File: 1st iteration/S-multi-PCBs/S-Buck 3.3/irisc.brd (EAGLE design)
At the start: 38.9 x 32.8 mm, 18 parts

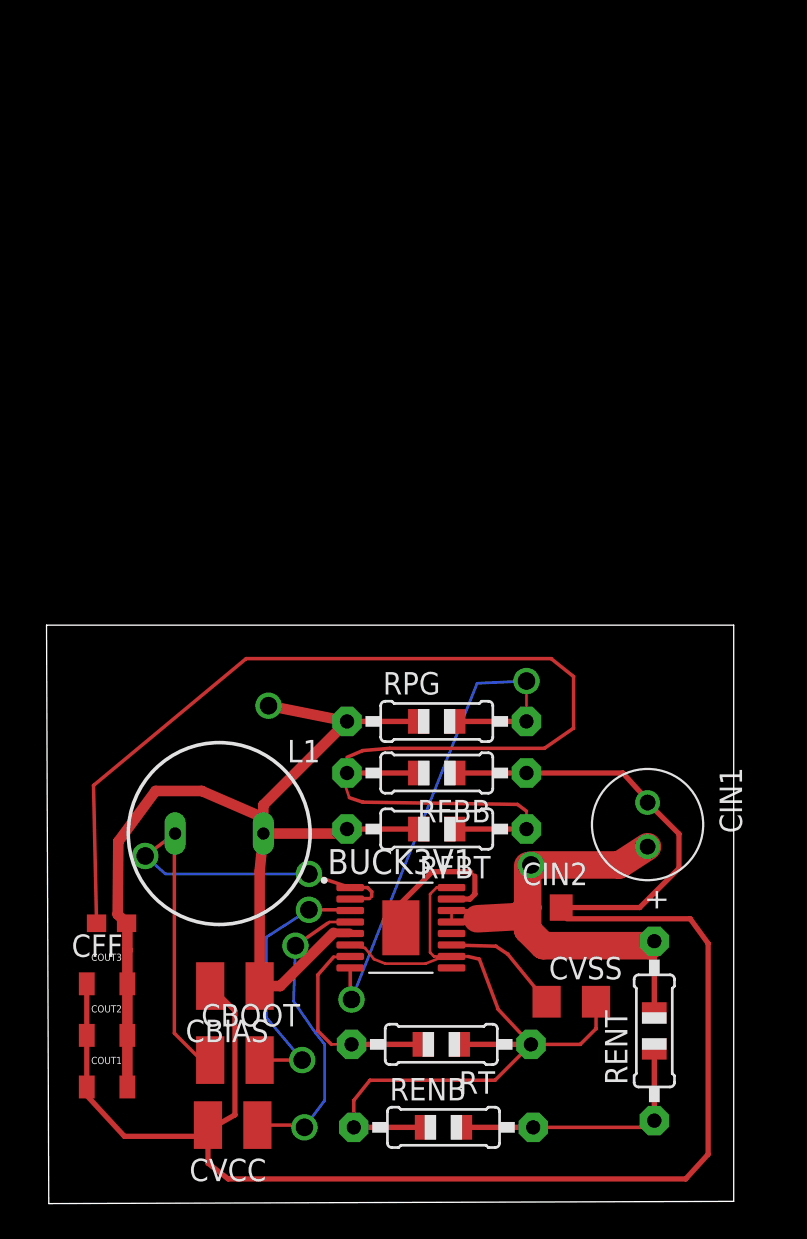
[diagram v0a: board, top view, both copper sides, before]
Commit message: Sabina Changes
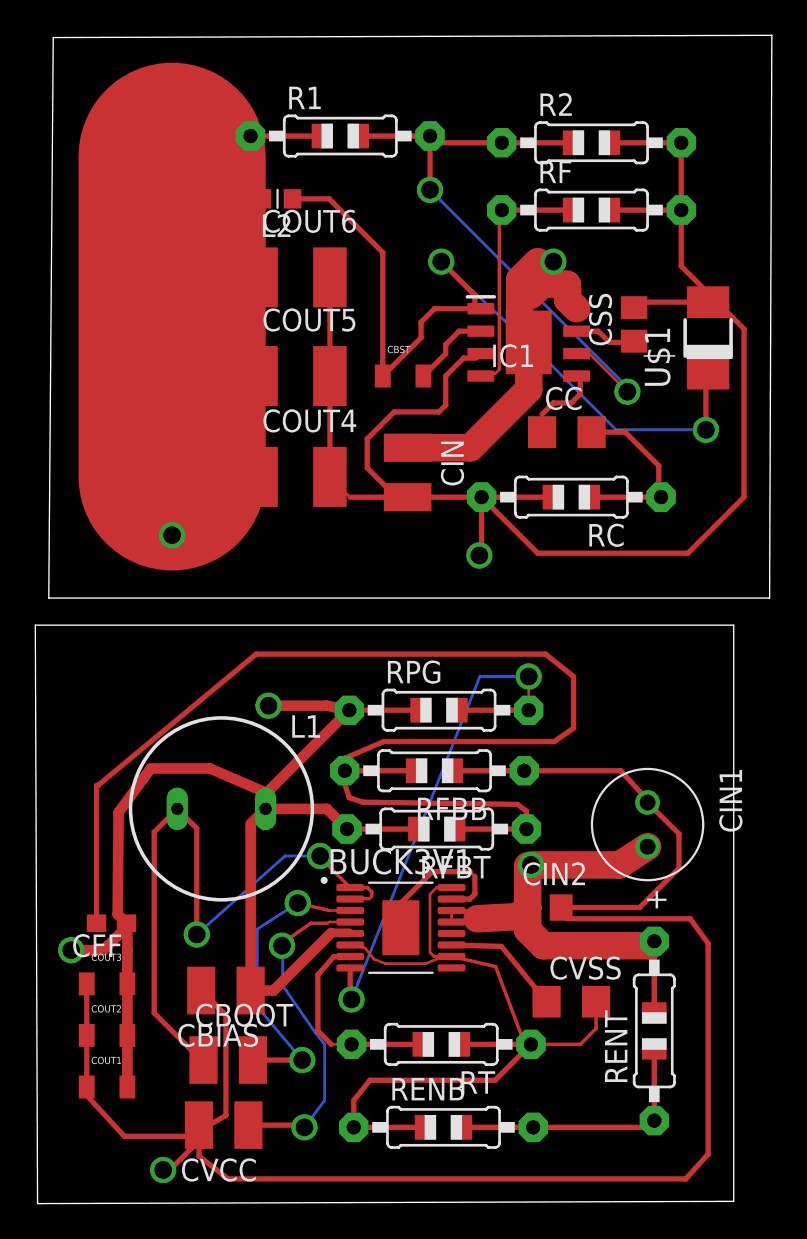
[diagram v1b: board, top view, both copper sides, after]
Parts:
- added CBST: 100 nF, Wurth_Elektronik_Passive_Capacitors_rev18b:WCAP-CSGP_0805_WAVE
- added CC: 1.44 pF, eagle-ltspice:C1206
- added CIN: 3 uF, eagle-ltspice:C1210
- added COUT4, COUT5, COUT6: 32 uF, eagle-ltspice:C1812
- added CSS: 850 pF, eagle-ltspice:C0805
- added IC1: AOZ1284PI, AOZ1284PI:SOIC127P600X170-9N
- added L2: 22uH, BeagleBone_Blue_R3:L0603
- added R1: 56 k, adafruit:0805-THM
- added R2: 10 k, adafruit:0805-THM
- added RC: 27 k, adafruit:0805-THM
- added RF: 270 k, adafruit:0805-THM
- added U$1: (no value), DO-214AC:DO-214AC
- moved L1 1.40 mm to (9.78, 22.4)
- moved RPG 0.65 mm to (22.1, 27.9)
- moved CBIAS 0.57 mm to (10.0, 12.1)
- moved CVCC 0.51 mm to (9.91, 4.45)
- moved CBOOT 0.38 mm to (10.2, 8.13)
- moved RFBB 0.18 mm to (21.8, 24.5)
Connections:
- new net 5V: COUT4.1, COUT5.1, COUT6.1, L2.2, R1.1
- new net N$11: CBST.2, IC1.2
- new net N$14: CBST.1, IC1.1, L2.1, U$1.C
- new net N$140: IC1.6, R1.2, R2.1
- new net N$141: CC.2, RC.1
- new net N$15: CC.1, IC1.5
- new net N$16: CSS.1, IC1.7
- new net N$5: IC1.4, RF.1
- new net VCC1: BUCK3V1.13, BUCK3V1.14, CIN1.1, CIN2.1, RENT.2
- net GND: now also CIN.2, COUT4.2, COUT5.2, COUT6.2, CSS.2, IC1.3, R2.2, RC.2, RF.2, U$1.A
- net VCC: now also CIN.1, IC1.8, IC1.9; no longer BUCK3V1.13, BUCK3V1.14, CIN1.1, CIN2.1, RENT.2
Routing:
- net GND: track 96.8 -> 180.4 mm, vias 0 -> 2
- net 5V: track 0.00 -> 58.9 mm, vias 0 -> 1
- net N$14: track 0.00 -> 46.7 mm, vias 0 -> 2
- net N$140: track 0.00 -> 27.0 mm, vias 0 -> 2
- net VCC1: track 0.00 -> 26.2 mm, vias 0 -> 1
- net N$5: track 0.00 -> 10.3 mm
- net 3.3V: track 59.1 -> 67.4 mm, vias 1 -> 2
- net N$1: track 31.1 -> 37.6 mm
- net N$141: track 0.00 -> 6.43 mm
- net N$15: track 0.00 -> 4.75 mm
- net N$11: track 0.00 -> 4.60 mm
- net N$16: track 0.00 -> 3.55 mm
- net VCC: track 26.2 -> 23.6 mm
- net N$4: track 15.3 -> 16.9 mm
- net N$12: track 17.5 -> 19.0 mm
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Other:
- board size 38.9 x 32.8 mm -> 41.7 x 66.2 mm
